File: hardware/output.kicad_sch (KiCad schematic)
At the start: 27 parts, among them J6 Conn_Coaxial, U19 ADL5611, U20 HMC624A, U21 ADL5611

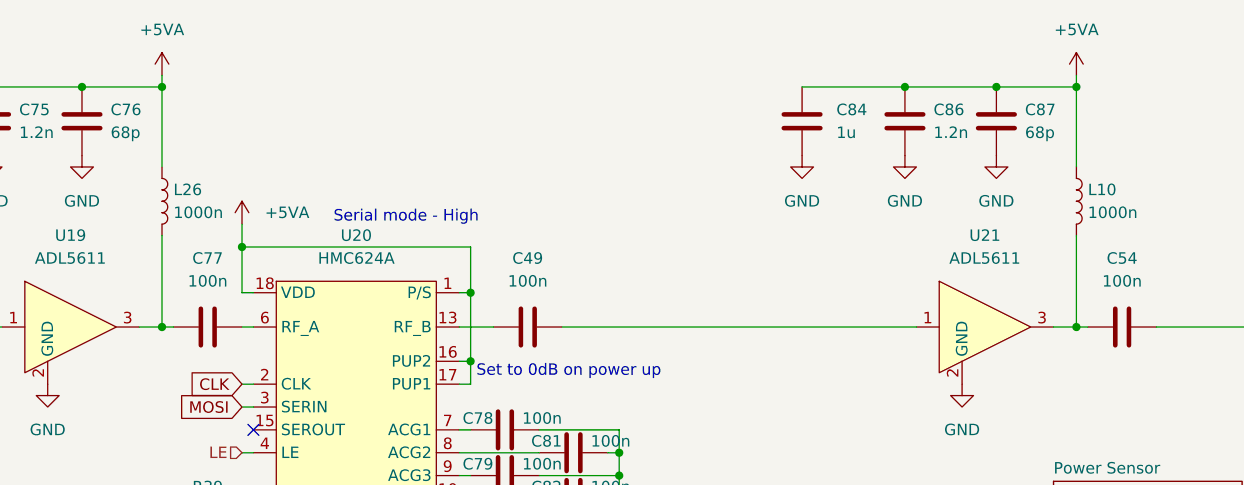
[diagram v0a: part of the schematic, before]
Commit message: FEM v3 Updates
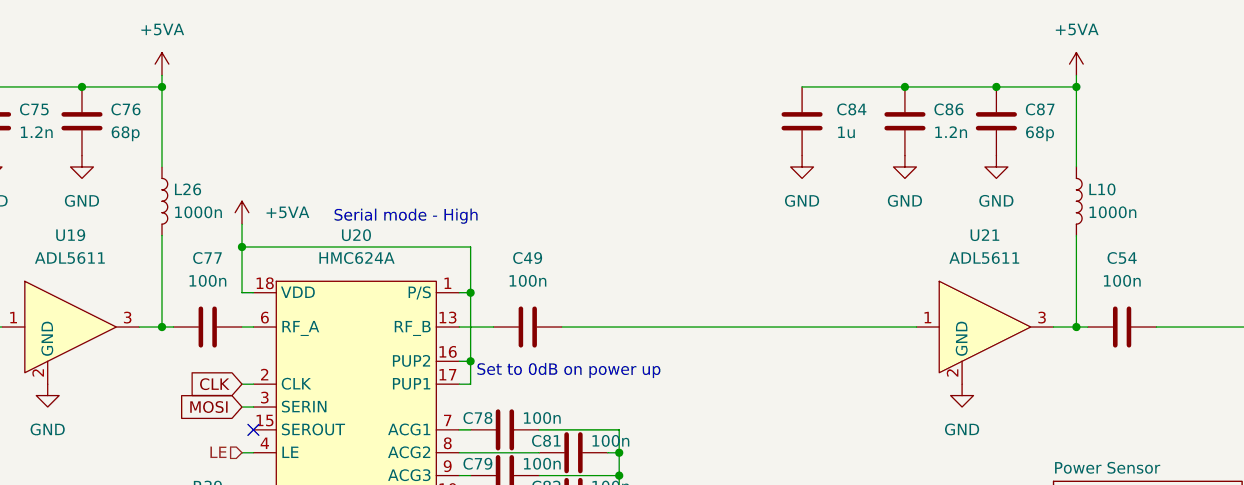
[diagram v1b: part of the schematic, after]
